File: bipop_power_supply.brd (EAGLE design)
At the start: 82.5 x 70.8 mm, 33 parts, among them IC1 LM1117MP-3.3, IC2 LM1117MP-5.0, X2 MSTBA6

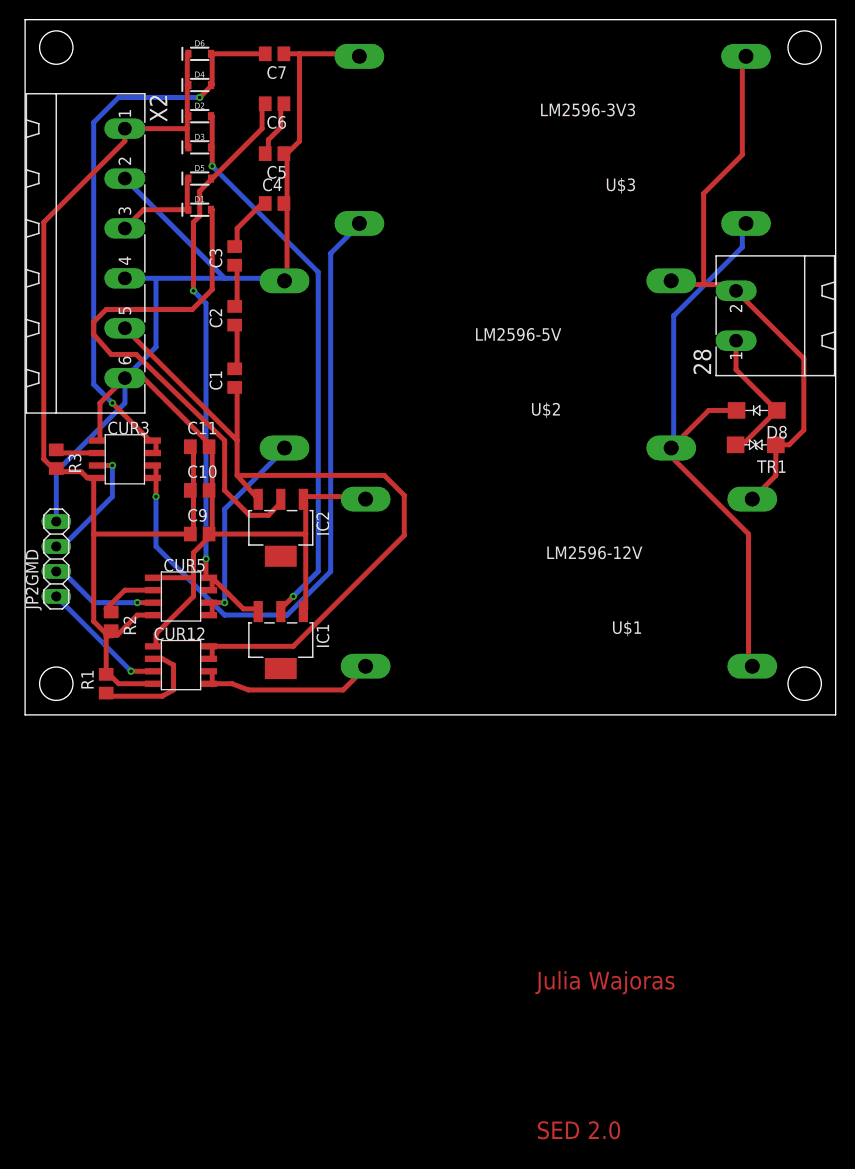
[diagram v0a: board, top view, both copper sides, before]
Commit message: small board adjustments, ready to gerber
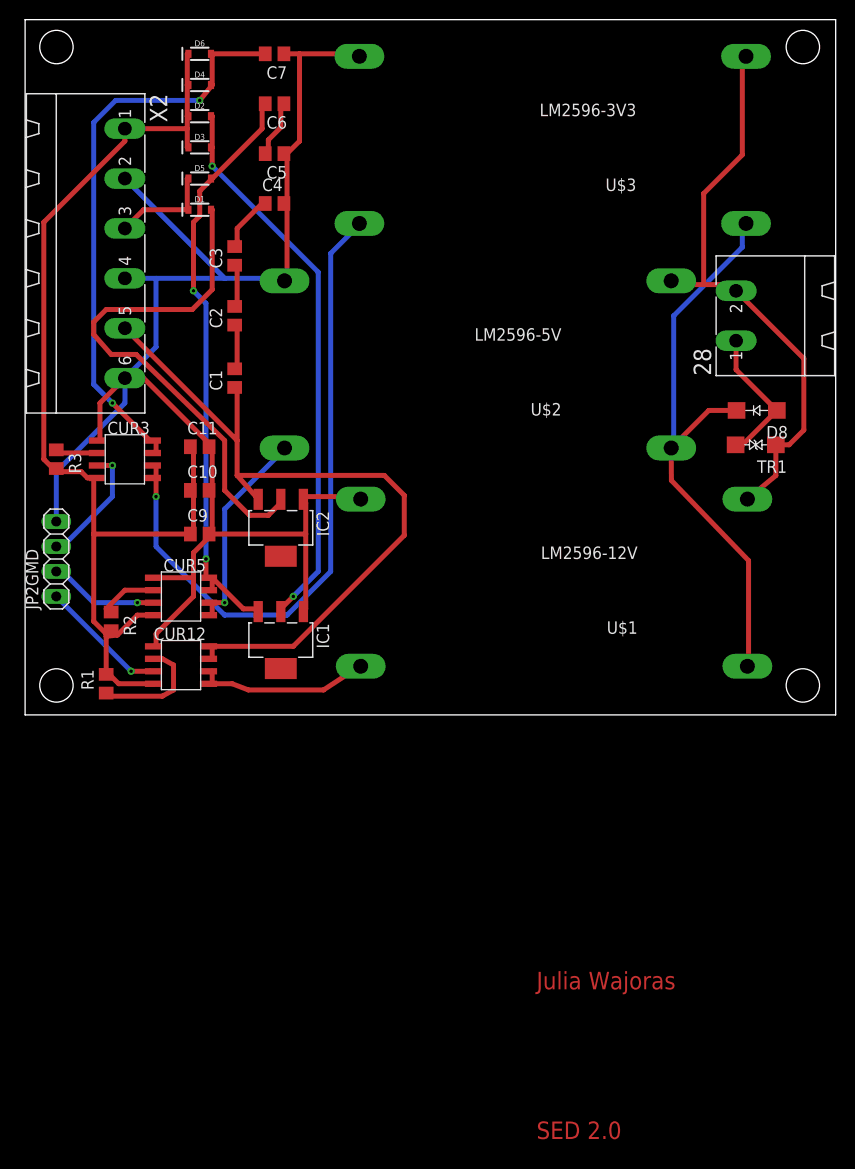
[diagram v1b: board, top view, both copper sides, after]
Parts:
- moved U$1 0.50 mm to (58.6, 13.3)
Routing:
- net 12_IN: track 18.8 -> 18.0 mm
- net MM: track 60.3 -> 59.7 mm
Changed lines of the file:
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@@
 <setting verticaltext="up"/>
 </settings>
-<grid distance="0.1" unitdist="mm" unit="mm" style="lines" multiple="1" display="yes" altdistance="5" altunitdist="mil" altunit="mil"/>
+<grid distance="0.5" unitdist="mm" unit="mm" style="lines" multiple="1" display="yes" altdistance="5" altunitdist="mil" altunit="mil"/>
 <layers>
 <layer number="1" name="Top" color="4" fill="1" visible="yes" active="yes"/>
@@
 <dimension x1="3.81" y1="0" x2="3.81" y2="70.79" x3="0" y3="35.395" textsize="1.778" layer="20" precision="1"/>
 <dimension x1="3.81" y1="70.79" x2="86.34" y2="70.79" x3="45.075" y3="73.66" textsize="1.778" layer="20" precision="1"/>
-<hole x="6.985" y="3.175" drill="3.39999375"/>
-<hole x="6.985" y="67.945" drill="3.39999375"/>
-<hole x="83.185" y="67.945" drill="3.39999375"/>
-<hole x="83.185" y="3.175" drill="3.39999375"/>
+<hole x="7" y="68" drill="3.4"/>
+<hole x="7" y="3" drill="3.4"/>
+<hole x="83" y="68" drill="3.4"/>
+<hole x="83" y="3" drill="3.4"/>
 </plain>
 <attributes>
@@
 <attribute name="PROD_ID" value="DIO-11623" x="21.59" y="67.31" size="1.778" layer="27" display="off"/>
 </element>
-<element name="U$1" library="lustro_pcb" package="DC-DC_CONVERTER" value="LM2596-12V" x="59.055" y="13.335" rot="R180"/>
+<element name="U$1" library="lustro_pcb" package="DC-DC_CONVERTER" value="LM2596-12V" x="58.555" y="13.335" rot="R180"/>
 <element name="U$2" library="lustro_pcb" package="DC-DC_CONVERTER" value="LM2596-5V" x="50.8" y="35.56" rot="R180"/>
 <element name="U$3" library="lustro_pcb" package="DC-DC_CONVERTER" value="LM2596-3V3" x="58.42" y="58.42" rot="R180"/>
@@
 <wire x1="32.385" y1="21.59" x2="32.145" y2="21.95" width="0.508" layer="1"/>
 <wire x1="32.385" y1="22.225" x2="38.1" y2="22.225" width="0.508" layer="1"/>
-<wire x1="38.1" y1="22.225" x2="38.481" y2="21.971" width="0.508" layer="1"/>
+<wire x1="38.1" y1="22.225" x2="37.981" y2="21.971" width="0.508" layer="1"/>
 <wire x1="32.385" y1="22.225" x2="32.145" y2="21.95" width="0.508" layer="1"/>
 <wire x1="22.86" y1="22.86" x2="22.86" y2="18.415" width="0.508" layer="1"/>
@@
 <wire x1="76.835" y1="66.675" x2="77.216" y2="67.056" width="0.508" layer="1"/>
 <contactref element="TR1" pad="P$1"/>
-<wire x1="77.851" y1="21.971" x2="80.25" y2="24.37" width="0.508" layer="1"/>
+<wire x1="77.351" y1="21.971" x2="80.25" y2="24.37" width="0.508" layer="1"/>
 <wire x1="80.25" y1="24.37" x2="80.25" y2="27.5" width="0.508" layer="1"/>
 <wire x1="80.25" y1="27.5" x2="81.6" y2="27.5" width="0.508" layer="1"/>
@@
 <wire x1="24.892" y1="3.175" x2="22.86" y2="3.175" width="0.508" layer="1"/>
 <wire x1="26.543" y1="2.54" x2="24.892" y2="3.175" width="0.508" layer="1"/>
-<wire x1="36.195" y1="2.54" x2="26.543" y2="2.54" width="0.508" layer="1"/>
-<wire x1="38.1" y1="4.445" x2="36.195" y2="2.54" width="0.508" layer="1"/>
+<wire x1="34.195" y1="2.54" x2="26.543" y2="2.54" width="0.508" layer="1"/>
+<wire x1="37.1" y1="4.445" x2="34.195" y2="2.54" width="0.508" layer="1"/>
 <wire x1="22.86" y1="3.175" x2="22.485" y2="3.17" width="0.508" layer="1"/>
-<wire x1="38.1" y1="4.445" x2="38.481" y2="4.953" width="0.508" layer="1"/>
+<wire x1="37.1" y1="4.445" x2="37.981" y2="4.953" width="0.508" layer="1"/>
 </signal>
 <signal name="3_OUT">
@@
 <wire x1="10.795" y1="33.655" x2="12.7" y2="31.75" width="0.508" layer="16"/>
 <wire x1="10.795" y1="60.325" x2="10.795" y2="33.655" width="0.508" layer="16"/>
-<wire x1="13.335" y1="62.865" x2="10.795" y2="60.325" width="0.508" layer="16"/>
-<wire x1="21.59" y1="62.865" x2="13.335" y2="62.865" width="0.508" layer="16"/>
-<wire x1="22.86" y1="64.135" x2="21.59" y2="62.865" width="0.508" layer="1"/>
+<wire x1="13.035" y1="62.565" x2="10.795" y2="60.325" width="0.508" layer="16"/>
+<wire x1="21.59" y1="62.565" x2="13.035" y2="62.565" width="0.508" layer="16"/>
+<wire x1="22.86" y1="64.135" x2="21.59" y2="62.565" width="0.508" layer="1"/>
 <wire x1="16.51" y1="27.94" x2="16.77" y2="27.935" width="0.508" layer="1"/>
 <wire x1="22.86" y1="64.135" x2="22.74" y2="64.135" width="0.508" layer="1"/>
 <via x="12.7" y="31.75" extent="1-16" drill="0.35"/>
-<via x="21.59" y="62.865" extent="1-16" drill="0.35"/>
+<via x="21.59" y="62.565" extent="1-16" drill="0.35"/>
 </signal>
 <signal name="VIOUT_3">
@@
 <contactref element="U$2" pad="V_IN+"/>
 <contactref element="U$3" pad="V_IN+"/>
-<wire x1="77.47" y1="18.415" x2="77.47" y2="5.08" width="0.508" layer="1"/>
-<wire x1="69.215" y1="26.67" x2="77.47" y2="18.415" width="0.508" layer="1"/>
-<wire x1="77.47" y1="5.08" x2="77.851" y2="4.953" width="0.508" layer="1"/>
-<wire x1="69.596" y1="27.178" x2="69.215" y2="26.67" width="0.508" layer="1"/>
+<wire x1="77.47" y1="15.715" x2="77.47" y2="5.08" width="0.508" layer="1"/>
+<wire x1="69.615" y1="23.87" x2="77.47" y2="15.715" width="0.508" layer="1"/>
+<wire x1="77.47" y1="5.08" x2="77.351" y2="4.953" width="0.508" layer="1"/>
+<wire x1="69.596" y1="27.178" x2="69.615" y2="23.87" width="0.508" layer="1"/>
 <wire x1="76.835" y1="47.625" x2="76.835" y2="49.53" width="0.508" layer="16"/>
 <wire x1="69.85" y1="40.64" x2="76.835" y2="47.625" width="0.508" layer="16"/>
